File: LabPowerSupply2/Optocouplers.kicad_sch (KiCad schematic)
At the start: 10 parts

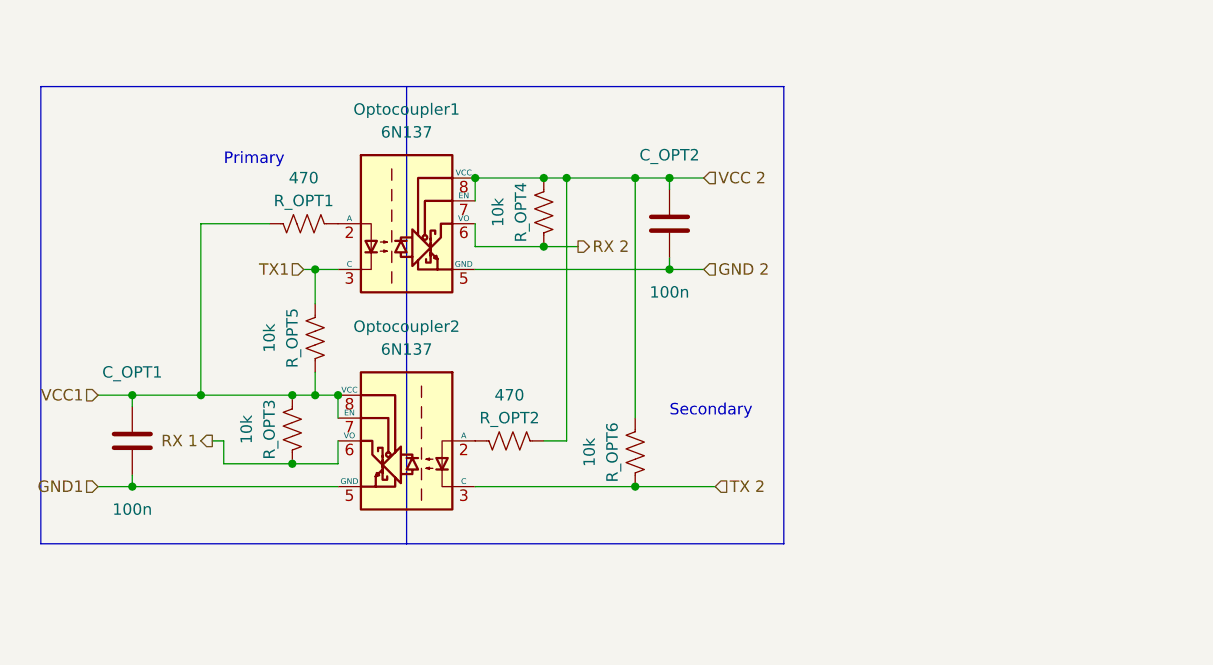
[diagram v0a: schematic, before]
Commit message: Beautifing the Schematic
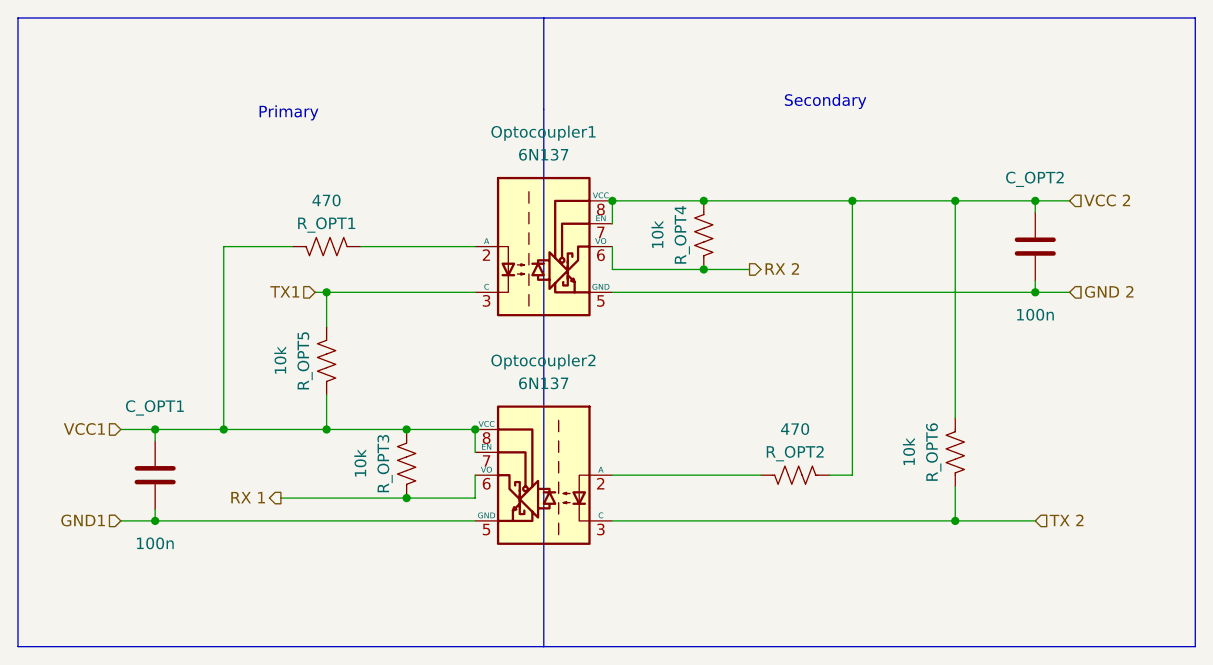
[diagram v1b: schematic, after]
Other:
- moved on the sheet: C_OPT1, C_OPT2, Optocoupler1, Optocoupler2, R_OPT1, R_OPT2, R_OPT3, R_OPT4, R_OPT5, R_OPT6
